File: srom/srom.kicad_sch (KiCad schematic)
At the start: 12 parts, among them J1 Conn_01x03_Female, U1 4075, U2 74LS245, U3 74LS245, U4 74LS245, U5 Pico-rp2040

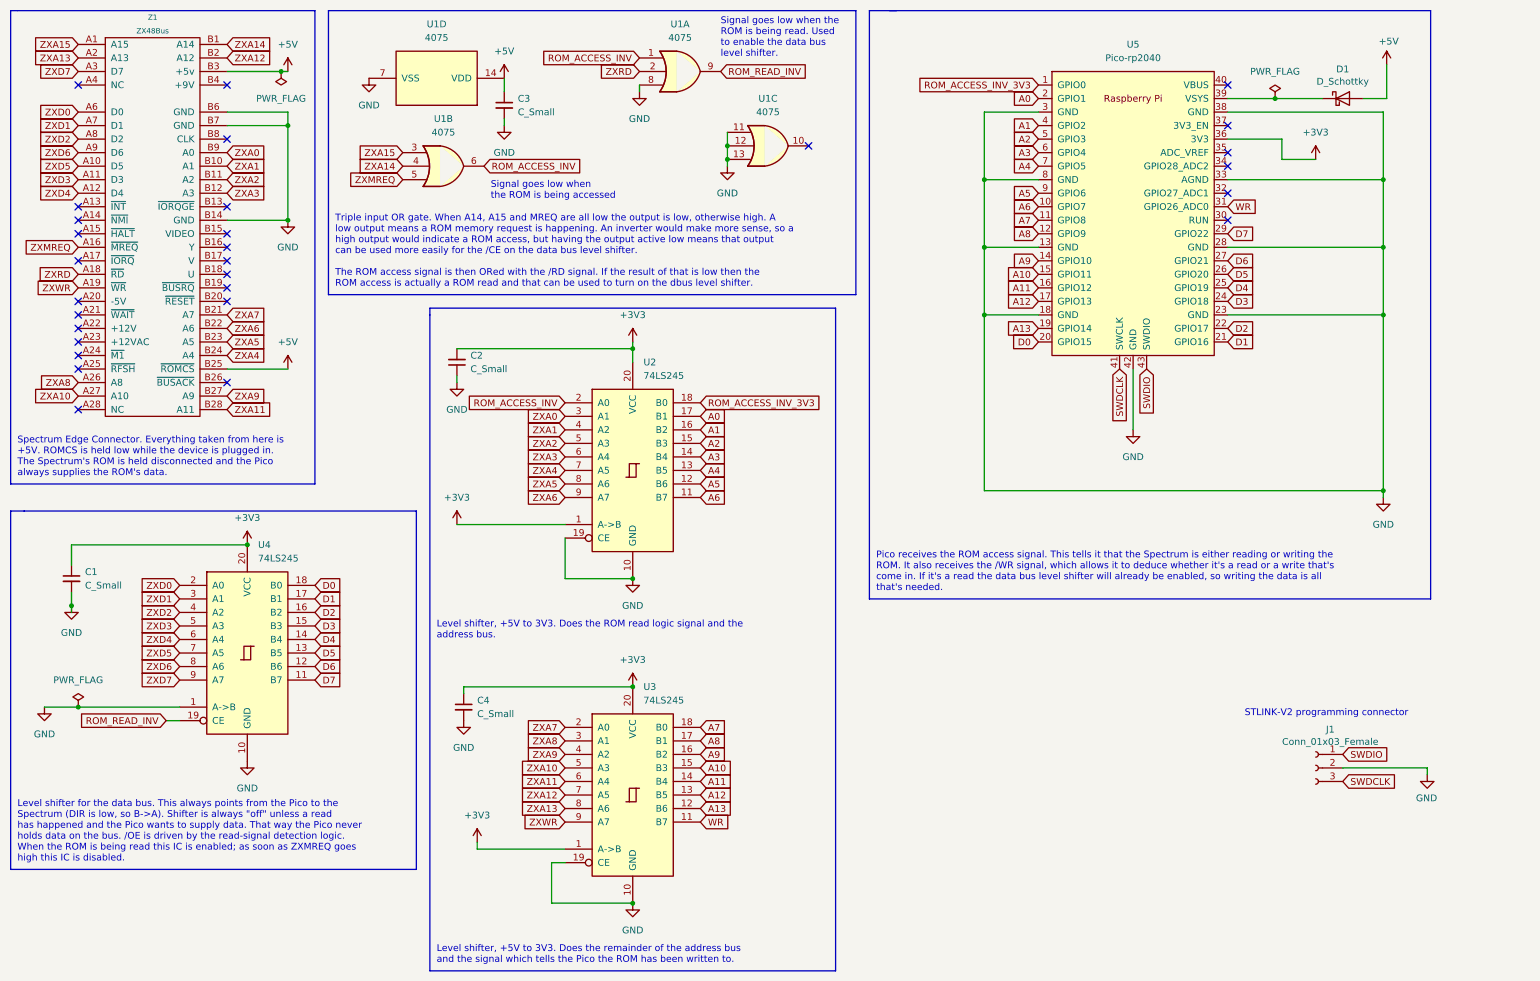
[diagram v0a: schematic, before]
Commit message: first effort at a layout
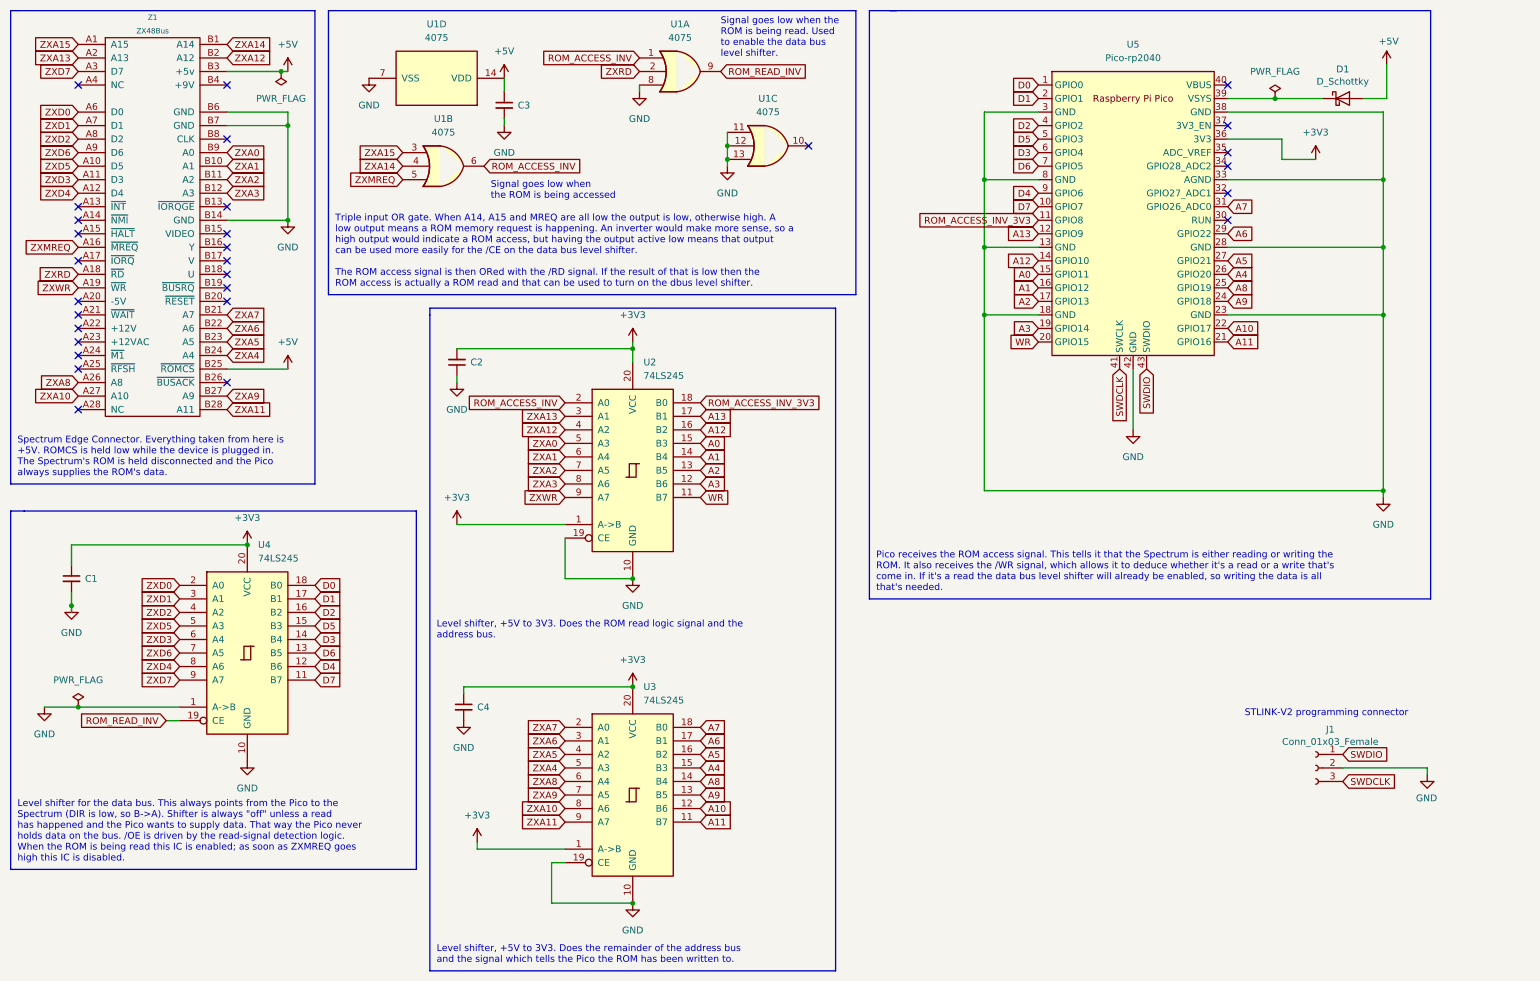
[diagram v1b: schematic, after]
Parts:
- U1: footprint (none) -> Package_SO:SOIC-14_3.9x8.7mm_P1.27mm
- U2, U3, U4: footprint (none) -> Package_SO:SOIC-20W_7.5x12.8mm_P1.27mm
- U5: footprint RPi_Pico:RPi_Pico_SMD_TH -> pico-foot:RPi_Pico_SMD_TH; symbol rp-pico:Pico-rp2040 -> pico-sym:Pico
- Z1: footprint (none) -> zxbus:ZX_Bus_Pin_Header
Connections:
- net A0: now also U2.15 (B3), U5.15 (GPIO11); no longer U2.17 (B1), U5.2 (GPIO1)
- net A1: now also U2.14 (B4), U5.16 (GPIO12); no longer U2.16 (B2), U5.4 (GPIO2)
- net A10: now also U3.12 (B6), U5.22 (GPIO17); no longer U3.15 (B3), U5.15 (GPIO11)
- net A11: now also U3.11 (B7), U5.21 (GPIO16); no longer U3.14 (B4), U5.16 (GPIO12)
- net A12: now also U2.16 (B2), U5.14 (GPIO10); no longer U3.13 (B5), U5.17 (GPIO13)
- net A13: now also U2.17 (B1), U5.12 (GPIO9); no longer U3.12 (B6), U5.19 (GPIO14)
- net A2: now also U2.13 (B5), U5.17 (GPIO13); no longer U2.15 (B3), U5.5 (GPIO3)
- net A3: now also U2.12 (B6), U5.19 (GPIO14); no longer U2.14 (B4), U5.6 (GPIO4)
- net A4: now also U3.15 (B3), U5.26 (GPIO20); no longer U2.13 (B5), U5.7 (GPIO5)
- net A5: now also U3.16 (B2), U5.27 (GPIO21); no longer U2.12 (B6), U5.9 (GPIO6)
- net A6: now also U3.17 (B1), U5.29 (GPIO22); no longer U2.11 (B7), U5.10 (GPIO7)
- net A7: now also U5.31 (GPIO26_ADC0); no longer U5.11 (GPIO8)
- net A8: now also U3.14 (B4), U5.25 (GPIO19); no longer U3.17 (B1), U5.12 (GPIO9)
- net A9: now also U3.13 (B5), U5.24 (GPIO18); no longer U3.16 (B2), U5.14 (GPIO10)
- net D0: now also U5.1 (GPIO0); no longer U5.20 (GPIO15)
- net D1: now also U5.2 (GPIO1); no longer U5.21 (GPIO16)
- net D2: now also U5.4 (GPIO2); no longer U5.22 (GPIO17)
- net D3: now also U4.14 (B4), U5.6 (GPIO4); no longer U4.15 (B3), U5.24 (GPIO18)
- net D4: now also U4.12 (B6), U5.9 (GPIO6); no longer U4.14 (B4), U5.25 (GPIO19)
- net D5: now also U4.15 (B3), U5.5 (GPIO3); no longer U4.13 (B5), U5.26 (GPIO20)
- net D6: now also U4.13 (B5), U5.7 (GPIO5); no longer U4.12 (B6), U5.27 (GPIO21)
- net D7: now also U5.10 (GPIO7); no longer U5.29 (GPIO22)
- net ROM_ACCESS_INV_3V3: now also U5.11 (GPIO8); no longer U5.1 (GPIO0)
- net WR: now also U2.11 (B7), U5.20 (GPIO15); no longer U3.11 (B7), U5.31 (GPIO26_ADC0)
- net ZXA0: now also U2.5 (A3); no longer U2.3 (A1)
- net ZXA1: now also U2.6 (A4); no longer U2.4 (A2)
- net ZXA10: now also U3.8 (A6); no longer U3.5 (A3)
- net ZXA11: now also U3.9 (A7); no longer U3.6 (A4)
- net ZXA12: now also U2.4 (A2); no longer U3.7 (A5)
- net ZXA13: now also U2.3 (A1); no longer U3.8 (A6)
- net ZXA2: now also U2.7 (A5); no longer U2.5 (A3)
- net ZXA3: now also U2.8 (A6); no longer U2.6 (A4)
- net ZXA4: now also U3.5 (A3); no longer U2.7 (A5)
- net ZXA5: now also U3.4 (A2); no longer U2.8 (A6)
- net ZXA6: now also U3.3 (A1); no longer U2.9 (A7)
- net ZXA8: now also U3.6 (A4); no longer U3.3 (A1)
- net ZXA9: now also U3.7 (A5); no longer U3.4 (A2)
- net ZXD3: now also U4.6 (A4); no longer U4.5 (A3)
- net ZXD4: now also U4.8 (A6); no longer U4.6 (A4)
- net ZXD5: now also U4.5 (A3); no longer U4.7 (A5)
- net ZXD6: now also U4.7 (A5); no longer U4.8 (A6)
- net ZXWR: now also U2.9 (A7); no longer U3.9 (A7)
